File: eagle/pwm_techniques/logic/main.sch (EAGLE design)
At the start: 52 parts, among them U1 LM2940T-10.0, U2 TLE2426ID, U3 LM358ADT

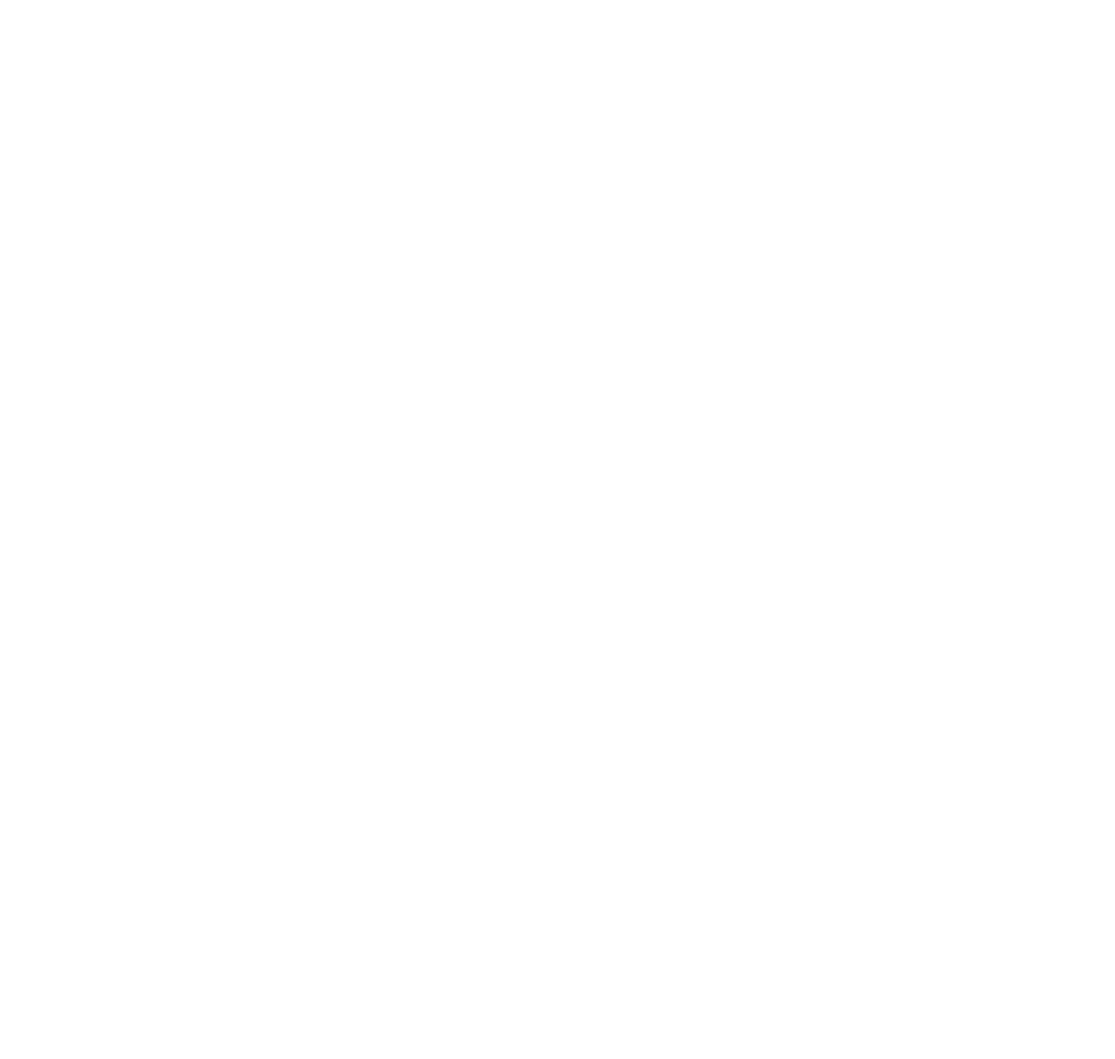
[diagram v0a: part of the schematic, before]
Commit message: [ update ] pwm control stage, wip
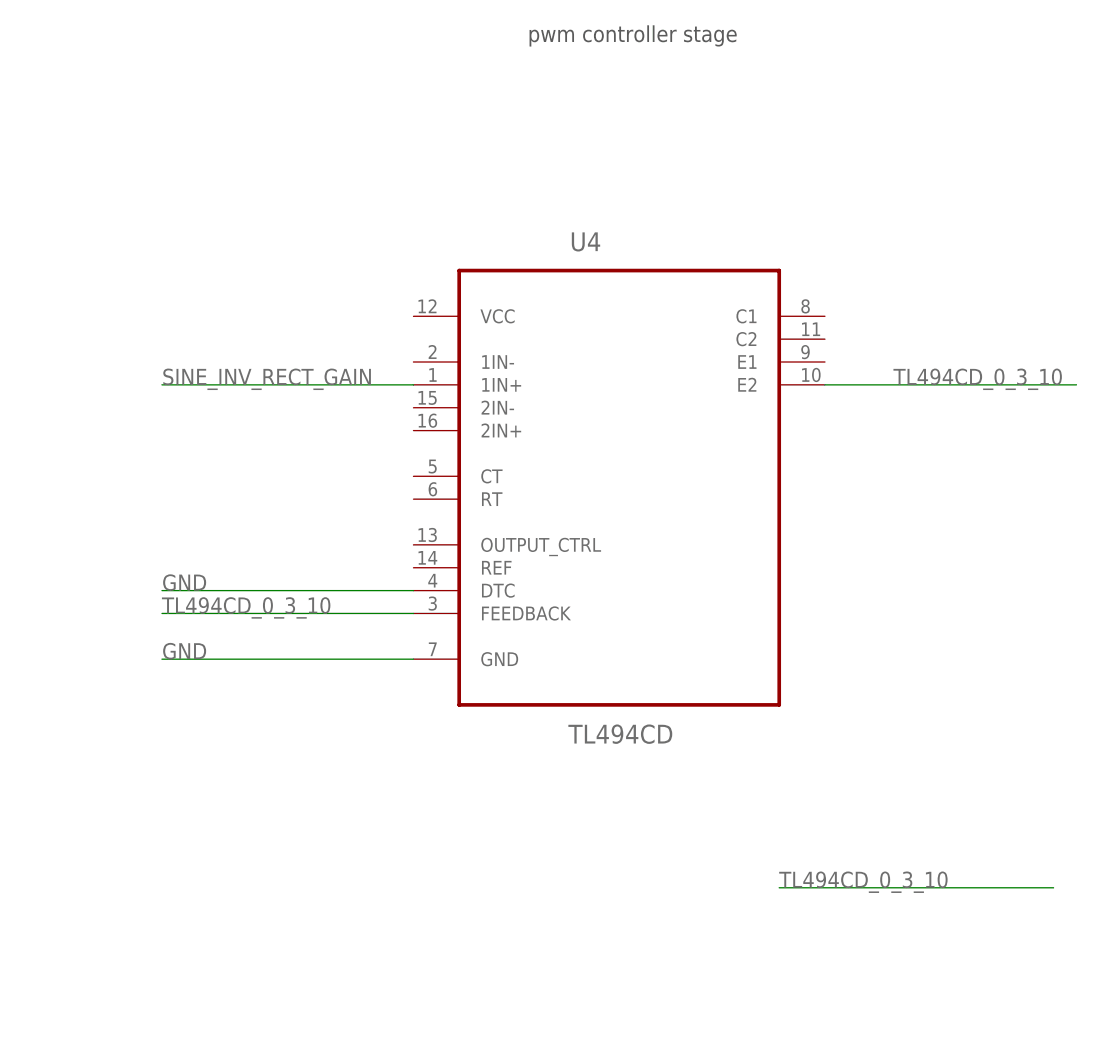
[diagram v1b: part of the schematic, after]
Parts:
- added U4: TL494CD, tl494cd:TL494CD
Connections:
- new net TL494CD_0_3_10: U4.E2, U4.FEEDBACK
- net GND: now also U4.DTC, U4.GND
- net SINE_INV_RECT_GAIN: now also U4.1IN+
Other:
- note added: "pwm controller stage"
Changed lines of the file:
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@@
 <part name="R21" library="resistor" deviceset="R-EU_" device="M1206" value="5K"/>
 <part name="R22" library="resistor" deviceset="R-EU_" device="M1206" value="20K"/>
+<part name="U4" library="tl494cd" deviceset="TL494CD" device=""/>
 </parts>
 <sheets>
@@
 <text x="228.6" y="101.6" size="1.778" layer="97">sine rect generation stage</text>
 <text x="322.58" y="101.6" size="1.778" layer="97">gain stage</text>
+<text x="454.66" y="101.6" size="1.778" layer="97">pwm controller stage</text>
 </plain>
 <instances>
@@
 <instance part="R21" gate="G$1" x="347.98" y="-12.7"/>
 <instance part="R22" gate="G$1" x="363.22" y="-12.7"/>
+<instance part="U4" gate="A" x="464.82" y="55.88"/>
 </instances>
 <busses>
@@
 <label x="375.92" y="-12.7" size="1.778" layer="95"/>
 </segment>
+<segment>
+<pinref part="U4" gate="A" pin="GND"/>
+<wire x1="441.96" y1="33.02" x2="414.02" y2="33.02" width="0.1524" layer="91"/>
+<label x="414.02" y="33.02" size="1.778" layer="95"/>
+</segment>
+<segment>
+<pinref part="U4" gate="A" pin="DTC"/>
+<wire x1="441.96" y1="40.64" x2="414.02" y2="40.64" width="0.1524" layer="91"/>
+<label x="414.02" y="40.64" size="1.778" layer="95"/>
+</segment>
 </net>
 <net name="VSPLIT_GND" class="0">
@@
 <label x="355.6" y="17.78" size="1.778" layer="95"/>
 </segment>
+<segment>
+<pinref part="U4" gate="A" pin="1IN+"/>
+<wire x1="441.96" y1="63.5" x2="414.02" y2="63.5" width="0.1524" layer="91"/>
+<label x="414.02" y="63.5" size="1.778" layer="95"/>
+</segment>
 </net>
 <net name="SINE_RECT_GAIN" class="0">
@@
 </segment>
 </net>
+<net name="TL494CD_0_3_10" class="0">
+<segment>
+<wire x1="482.6" y1="7.62" x2="513.08" y2="7.62" width="0.1524" layer="91"/>
+<label x="482.6" y="7.62" size="1.778" layer="95"/>
+</segment>
+<segment>
+<wire x1="414.02" y1="38.1" x2="441.96" y2="38.1" width="0.1524" layer="91"/>
+<label x="414.02" y="38.1" size="1.778" layer="95"/>
+<pinref part="U4" gate="A" pin="FEEDBACK"/>
+</segment>
+<segment>
+<wire x1="487.68" y1="63.5" x2="515.62" y2="63.5" width="0.1524" layer="91"/>
+<label x="495.3" y="63.5" size="1.778" layer="95"/>
+<pinref part="U4" gate="A" pin="E2"/>
+</segment>
+</net>
